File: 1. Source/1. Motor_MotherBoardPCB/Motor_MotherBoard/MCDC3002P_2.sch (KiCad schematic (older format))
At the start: 3 parts, among them U6 MCDC3002P, U7 CON_6pin_motor

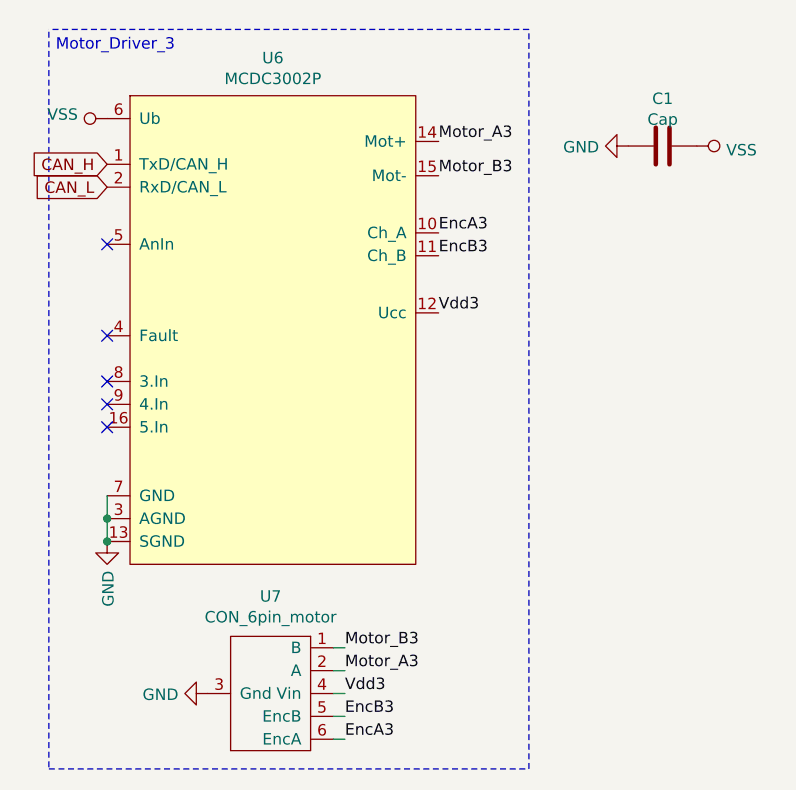
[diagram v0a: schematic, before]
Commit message: PCB_MotorMotherBoard
PCB_MotorMotherBoard
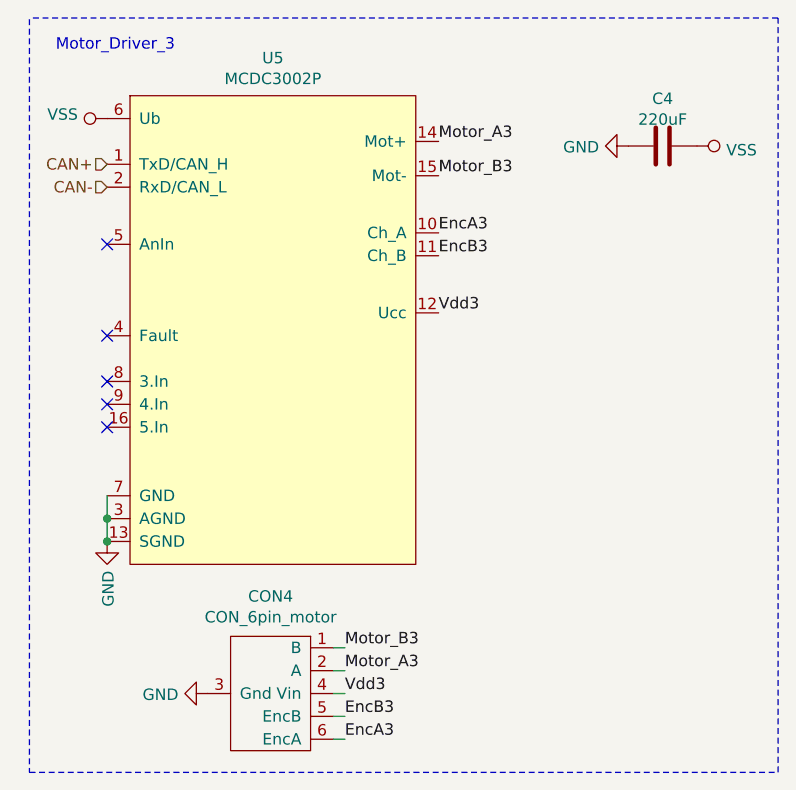
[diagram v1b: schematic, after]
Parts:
- removed C1: Cap, Capacitor_THT:CP_Radial_D6.3mm_P2.50mm, symbol Device:C
- removed U6: MCDC3002P, BC_Motor_Driver:MCDC_3002P, symbol BC_Motor_Drivers:MCDC3002P
- removed U7: CON_6pin_motor, Connector_IDC:IDC-Header_2x03_P2.54mm_Vertical, symbol BC_Connectors:CON_6pin_motor
- added C4: 220uF, Capacitor_THT:CP_Radial_D8.0mm_P3.50mm, symbol Device:C
- added CON4: CON_6pin_motor, Connector_IDC:IDC-Header_2x03_P2.54mm_Vertical, symbol BC_Connectors:CON_6pin_motor
- added U5: MCDC3002P, BC_Motor_Driver:MCDC_3002P, symbol BC_Motor_Drivers:MCDC3002P
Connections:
- net EncA3: now also CON4.6 (EncA), U5.10 (Ch_A)
- net EncB3: now also CON4.5 (EncB), U5.11 (Ch_B)
- net GND: now also C4.2, CON4.3 (Gnd), U5.13 (SGND), U5.3 (AGND), U5.7 (GND)
- net Motor_A3: now also CON4.2 (A), U5.14 (Mot+)
- net Motor_B3: now also CON4.1 (B), U5.15 (Mot-)
- net VSS: now also C4.1, U5.6 (Ub)
- net Vdd3: now also CON4.4 (Vin), U5.12 (Ucc)
- new net CAN+: U5.1 (TxD/CAN_H)
- new net CAN-: U5.2 (RxD/CAN_L)
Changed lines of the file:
@@
 $EndDescr
 $Comp
-L BC_Motor_Drivers:MCDC3002P U6
-U 1 1 6362D407
+L BC_Motor_Drivers:MCDC3002P U5
+U 1 1 6383589F
 P 4625 2850
-F 0 "U6" H 4650 4015 50  0000 C CNN
+F 0 "U5" H 4650 4015 50  0000 C CNN
 F 1 "MCDC3002P" H 4650 3924 50  0000 C CNN
 F 2 "BC_Motor_Driver:MCDC_3002P" H 5075 2550 50  0001 C CNN
@@
 $EndComp
 $Comp
-L BC_Connectors:CON_6pin_motor U7
-U 1 1 6362D408
+L BC_Connectors:CON_6pin_motor CON4
+U 1 1 638358A0
 P 4665 4465
-F 0 "U7" V 4240 4440 50  0000 C CNN
+F 0 "CON4" V 4240 4440 50  0000 C CNN
 F 1 "CON_6pin_motor" V 4331 4440 50  0000 C CNN
 F 2 "Connector_IDC:IDC-Header_2x03_P2.54mm_Vertical" H 4665 4565 50  0001 C CNN
@@
 	4915 4265 4965 4265
 $Comp
-L power:GND #PWR021
+L power:GND #PWR0121
 U 1 1 6362D409
 P 4365 4465
-F 0 "#PWR021" H 4365 4215 50  0001 C CNN
+F 0 "#PWR0121" H 4365 4215 50  0001 C CNN
 F 1 "GND" V 4370 4337 50  0000 R CNN
 F 2 "" H 4365 4465 50  0001 C CNN
@@
 	3925 3700 3925 3800
 $Comp
-L power:GND #PWR020
+L power:GND #PWR0122
 U 1 1 6362D40A
 P 3925 3800
-F 0 "#PWR020" H 3925 3550 50  0001 C CNN
+F 0 "#PWR0122" H 3925 3550 50  0001 C CNN
 F 1 "GND" V 3930 3672 50  0000 R CNN
 F 2 "" H 3925 3800 50  0001 C CNN
@@
 NoConn ~ 3925 3300
 Connection ~ 3925 3800
-Wire Notes Line
-	3670 1570 3670 4795
-Wire Notes Line
-	3670 4795 5770 4795
-Wire Notes Line
-	5770 4795 5770 1560
-Wire Notes Line
-	5770 1560 3670 1560
 Text Notes 3700 1660 0    50   ~ 0
 Motor_Driver_3\n
@@
 Wire Wire Line
 	4915 4365 4965 4365
-Text GLabel 3925 2150 0    50   Input ~ 0
-CAN_H
-Text GLabel 3925 2250 0    50   Input ~ 0
-CAN_L
 $Comp
 L Device:C R?
-U 1 1 6362C896
+U 1 1 6383589B
 P 6355 2070
-AR Path="/635EAE14/6362C896" Ref="R?"  Part="1"
-AR Path="/6360DF7C/6362C896" Ref="R?"  Part="1"
-AR Path="/6362A5B1/6362C896" Ref="C1"  Part="1"
-F 0 "C1" V 6148 2070 50  0000 C CNN
-F 1 "Cap" V 6239 2070 50  0000 C CNN
-F 2 "Capacitor_THT:CP_Radial_D6.3mm_P2.50mm" V 6285 2070 50  0001 C CNN
+AR Path="/635EAE14/6383589B" Ref="R?"  Part="1"
+AR Path="/6360DF7C/6383589B" Ref="R?"  Part="1"
+AR Path="/6362A5B1/6383589B" Ref="C4"  Part="1"
+F 0 "C4" V 6148 2070 50  0000 C CNN
+F 1 "220uF" V 6239 2070 50  0000 C CNN
+F 2 "Capacitor_THT:CP_Radial_D8.0mm_P3.50mm" V 6285 2070 50  0001 C CNN
 F 3 "~" H 6355 2070 50  0001 C CNN
 	1    6355 2070
@@
 $Comp
 L power:VSS #PWR?
-U 1 1 6362C89C
+U 1 1 6383589C
 P 6505 2070
-AR Path="/635EAE14/6362C89C" Ref="#PWR?"  Part="1"
-AR Path="/6360DF7C/6362C89C" Ref="#PWR?"  Part="1"
-AR Path="/6362A5B1/6362C89C" Ref="#PWR018"  Part="1"
-F 0 "#PWR018" H 6505 1920 50  0001 C CNN
+AR Path="/635EAE14/6383589C" Ref="#PWR?"  Part="1"
+AR Path="/6360DF7C/6383589C" Ref="#PWR?"  Part="1"
+AR Path="/6362A5B1/6383589C" Ref="#PWR0123"  Part="1"
+F 0 "#PWR0123" H 6505 1920 50  0001 C CNN
 F 1 "VSS" V 6523 2198 50  0000 L CNN
 F 2 "" H 6505 2070 50  0001 C CNN
@@
 $Comp
 L power:GND #PWR?
-U 1 1 6362C8A2
+U 1 1 6383589D
 P 6205 2070
-AR Path="/635EAE14/6362C8A2" Ref="#PWR?"  Part="1"
-AR Path="/6360DF7C/6362C8A2" Ref="#PWR?"  Part="1"
-AR Path="/6362A5B1/6362C8A2" Ref="#PWR019"  Part="1"
-F 0 "#PWR019" H 6205 1820 50  0001 C CNN
+AR Path="/635EAE14/6383589D" Ref="#PWR?"  Part="1"
+AR Path="/6360DF7C/6383589D" Ref="#PWR?"  Part="1"
+AR Path="/6362A5B1/6383589D" Ref="#PWR0124"  Part="1"
+F 0 "#PWR0124" H 6205 1820 50  0001 C CNN
 F 1 "GND" V 6210 1942 50  0000 R CNN
 F 2 "" H 6205 2070 50  0001 C CNN
@@
 $Comp
 L power:VSS #PWR?
-U 1 1 6362C93C
+U 1 1 6383589E
 P 3925 1950
-AR Path="/635EAE14/6362C93C" Ref="#PWR?"  Part="1"
-AR Path="/6360DF7C/6362C93C" Ref="#PWR?"  Part="1"
-AR Path="/6362A5B1/6362C93C" Ref="#PWR017"  Part="1"
-F 0 "#PWR017" H 3925 1800 50  0001 C CNN
+AR Path="/635EAE14/6383589E" Ref="#PWR?"  Part="1"
+AR Path="/6360DF7C/6383589E" Ref="#PWR?"  Part="1"
+AR Path="/6362A5B1/6383589E" Ref="#PWR0125"  Part="1"
+F 0 "#PWR0125" H 3925 1800 50  0001 C CNN
 F 1 "VSS" V 3943 2078 50  0000 L CNN
 F 2 "" H 3925 1950 50  0001 C CNN
@@
 	0    -1   -1   0
 $EndComp
+Text HLabel 3925 2150 0    50   Input ~ 0
+CAN+
+Text HLabel 3925 2250 0    50   Input ~ 0
+CAN-
+Wire Notes Line
+	3585 1515 3585 4810
+Wire Notes Line
+	3585 4810 6860 4810
+Wire Notes Line
+	6860 4810 6860 1510
+Wire Notes Line
+	6860 1510 3585 1510
 $EndSCHEMATC
